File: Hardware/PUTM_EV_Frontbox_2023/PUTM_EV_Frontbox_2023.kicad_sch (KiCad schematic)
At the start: 18 parts, among them J1 Conn_02x16_Counter_Clockwise, J2 Conn_01x04, SW1 Reset switch, U1 STM32G473RCTx

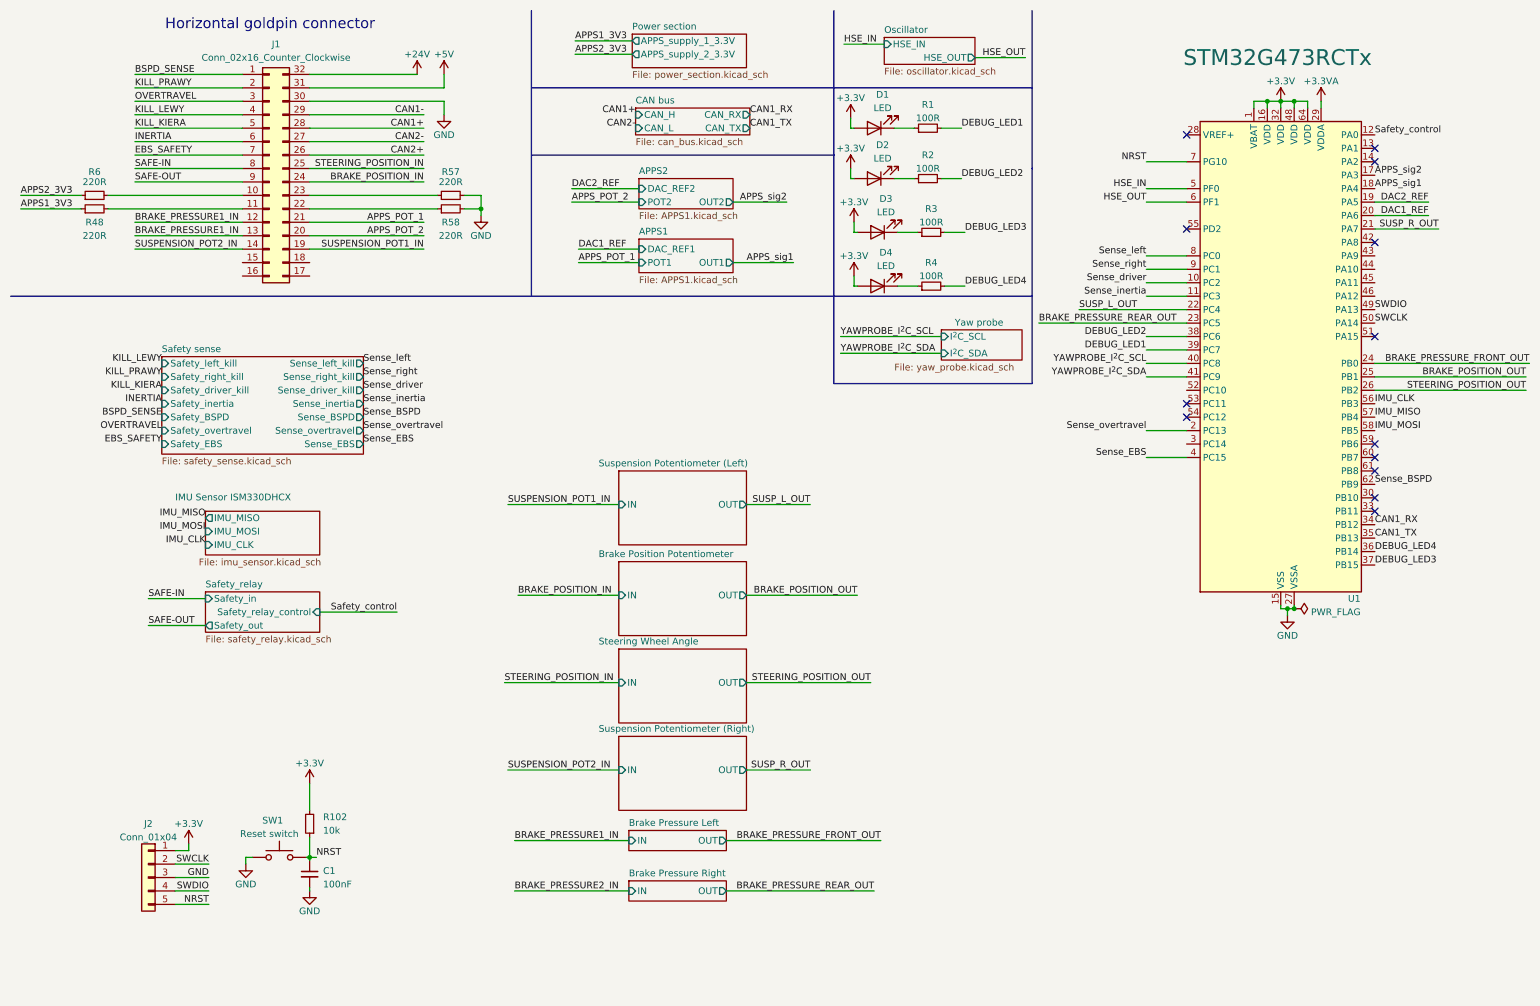
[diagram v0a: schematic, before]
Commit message: Started PCB layout
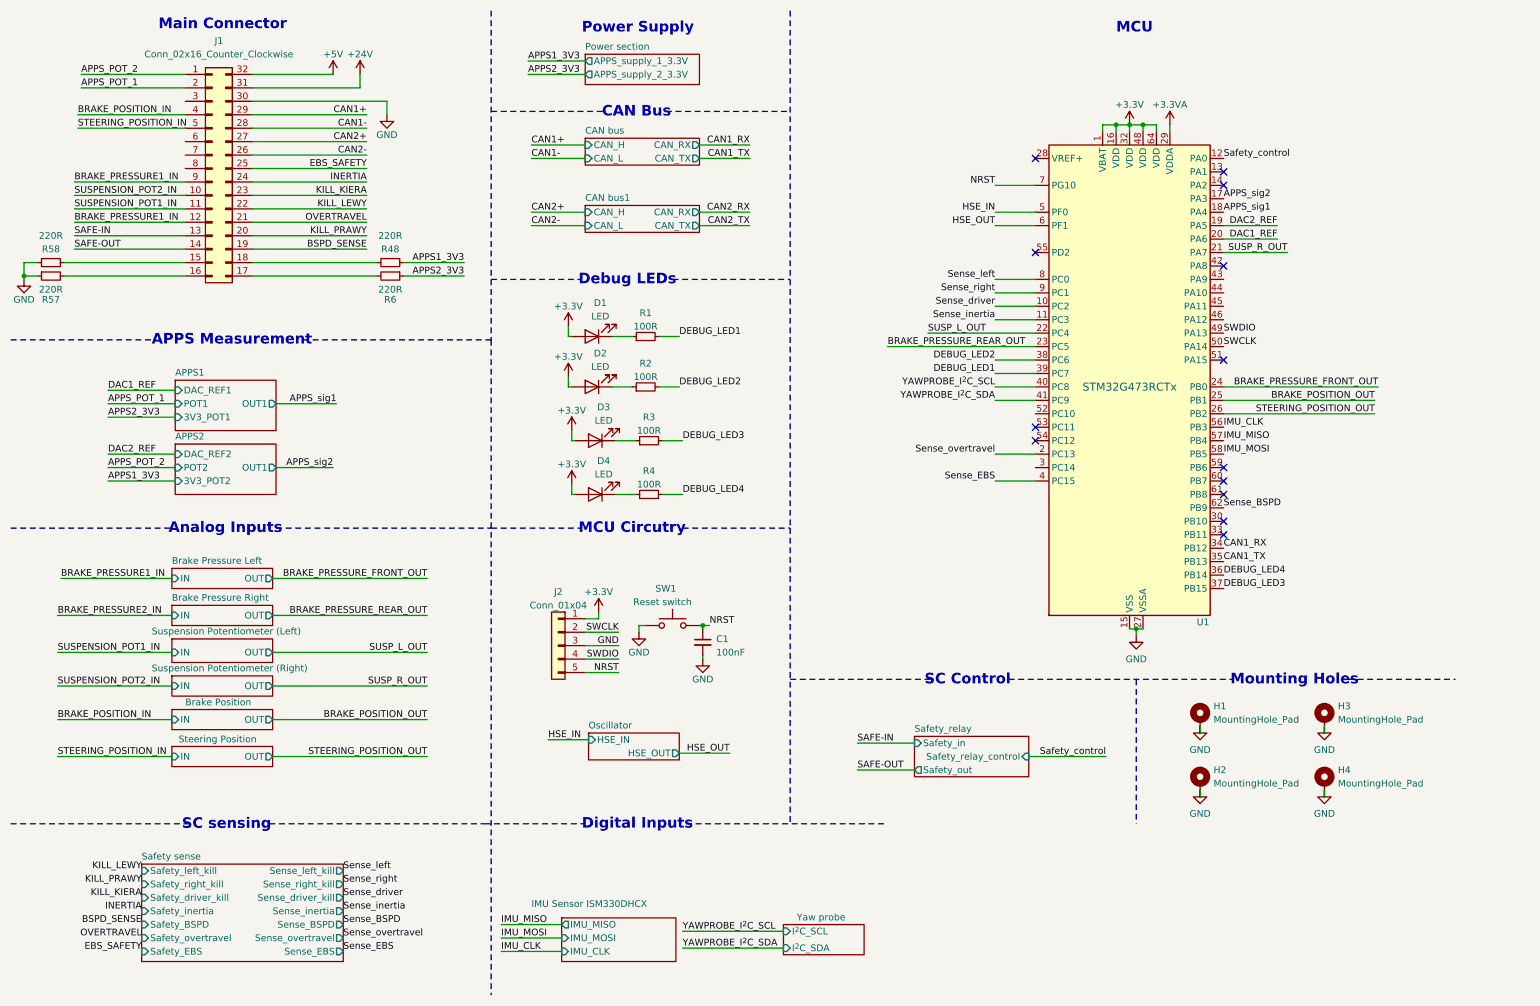
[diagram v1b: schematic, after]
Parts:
- removed R102: 10k, Resistor_SMD:R_0603_1608Metric_Pad0.98x0.95mm_HandSolder, symbol Device:R_Small
- added H1, H2, H3, H4: MountingHole_Pad, MountingHole:MountingHole_3.2mm_M3_DIN965_Pad_TopBottom, symbol Mechanical:MountingHole_Pad
- J1: footprint (none) -> Connector_PinHeader_2.54mm:PinHeader_2x16_P2.54mm_Vertical
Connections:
- net +24V: now also J1.31 (Pin_31); no longer J1.32 (Pin_32)
- net +5V: now also J1.32 (Pin_32); no longer J1.31 (Pin_31)
- net APPS_POT_1: now also J1.2 (Pin_2); no longer J1.21 (Pin_21)
- net APPS_POT_2: now also J1.1 (Pin_1); no longer J1.20 (Pin_20)
- net BRAKE_POSITION_IN: now also J1.4 (Pin_4); no longer J1.24 (Pin_24)
- net BRAKE_PRESSURE1_IN: now also J1.9 (Pin_9); no longer J1.13 (Pin_13)
- net BSPD_SENSE: now also J1.19 (Pin_19); no longer J1.1 (Pin_1)
- net CAN1+: now also J1.29 (Pin_29); no longer J1.28 (Pin_28)
- net CAN1-: now also J1.28 (Pin_28); no longer J1.29 (Pin_29)
- net CAN2+: now also J1.27 (Pin_27); no longer J1.26 (Pin_26)
- net CAN2-: now also J1.26 (Pin_26); no longer J1.27 (Pin_27)
- net EBS_SAFETY: now also J1.25 (Pin_25); no longer J1.7 (Pin_7)
- net GND: now also R57.1, R58.1, H1.1, H2.1, H3.1, H4.1; no longer R57.2, R58.2
- net INERTIA: now also J1.24 (Pin_24); no longer J1.6 (Pin_6)
- net KILL_KIERA: now also J1.23 (Pin_23); no longer J1.5 (Pin_5)
- net KILL_LEWY: now also J1.22 (Pin_22); no longer J1.4 (Pin_4)
- net KILL_PRAWY: now also J1.20 (Pin_20); no longer J1.2 (Pin_2)
- net OVERTRAVEL: now also J1.21 (Pin_21); no longer J1.3 (Pin_3)
- net SAFE-IN: now also J1.13 (Pin_13); no longer J1.8 (Pin_8)
- net SAFE-OUT: now also J1.14 (Pin_14); no longer J1.9 (Pin_9)
- net STEERING_POSITION_IN: now also J1.5 (Pin_5); no longer J1.25 (Pin_25)
- net SUSPENSION_POT1_IN: now also J1.11 (Pin_11); no longer J1.19 (Pin_19)
- net SUSPENSION_POT2_IN: now also J1.10 (Pin_10); no longer J1.14 (Pin_14)
- net at R48.2: now also J1.18 (Pin_18); no longer J1.11 (Pin_11)
- net at R6.2: now also J1.17 (Pin_17); no longer J1.10 (Pin_10)
- net at J1.15 (Pin_15): now also R58.2
- net at J1.16 (Pin_16): now also R57.2
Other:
- removed sheet Brake Position Potentiometer
- removed sheet Steering Wheel Angle
- added sheet Brake Position (suspension_potentiometer.kicad_sch)
- added sheet CAN bus1 (can_bus.kicad_sch)
- added sheet Steering Position (suspension_potentiometer.kicad_sch)
- sheet APPS1 ports: added 3V3_POT1; removed none
- sheet APPS2: file APPS1.kicad_sch -> APPS2.kicad_sch
- sheet APPS2 ports: added 3V3_POT2, OUT1; removed OUT2
- note added: "APPS Measurement"
- note added: "Analog Inputs"
- note added: "CAN Bus"
- note added: "Debug LEDs"
- note added: "Digital Inputs"
- note added: "MCU"
- note added: "MCU Circutry"
- note added: "Main Connector"
- note added: "Mounting Holes"
- note added: "Power Supply"
- note added: "SC Control"
- note added: "SC sensing"
- note removed: "Horizontal goldpin connector"
- company: Author: Szymon Kostrubiec -> Author: Adam Wasilewski
- moved on the sheet: C1, D1, D2, D3, D4, J2, R1, R2, R3, R4, R48, R57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
